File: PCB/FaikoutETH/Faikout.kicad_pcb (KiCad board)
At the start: 2 copper layers, 70 x 70 mm, 70 parts, among them J1 1x5, J2 TC2030-USB-NL, J3 Reset, J4 RJ45_LED, Q1 BSS138PS, U1 KSZ8851SNL, U4 ESP32-S3-MINI-1, U5 TPS62933, Y1 Crystal_GND24

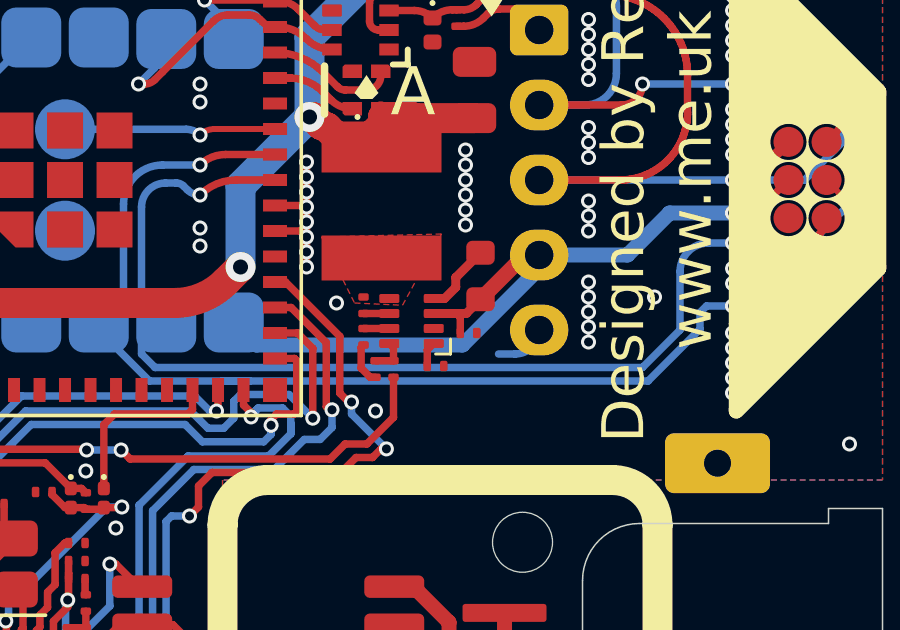
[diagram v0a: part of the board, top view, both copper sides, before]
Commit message: Tidy
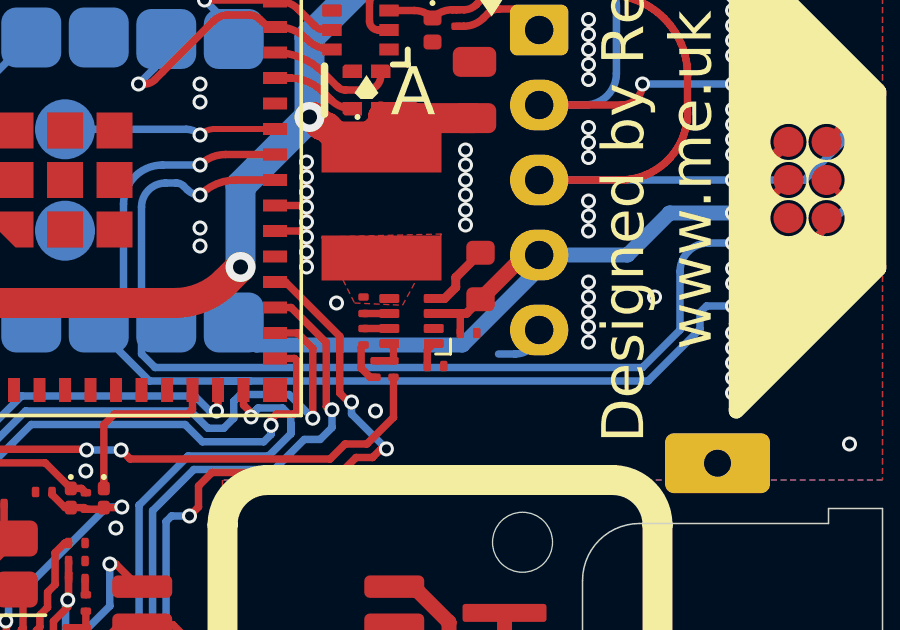
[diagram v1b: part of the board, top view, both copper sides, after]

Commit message: Re-render, latest layout
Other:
- board text added: "5 V-cuts"
- board text removed: "6 V-cuts"
